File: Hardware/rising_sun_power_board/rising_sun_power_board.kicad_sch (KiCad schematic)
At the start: 30 parts, among them J1 POWER_IN, J2 Conn_01x03_Socket, J3 Conn_01x03_Socket, SW201 SW_Push, U1 ESP32, U2 MIC5219, U3 UA78M05IDCYR, U4 TXU0102DCUR

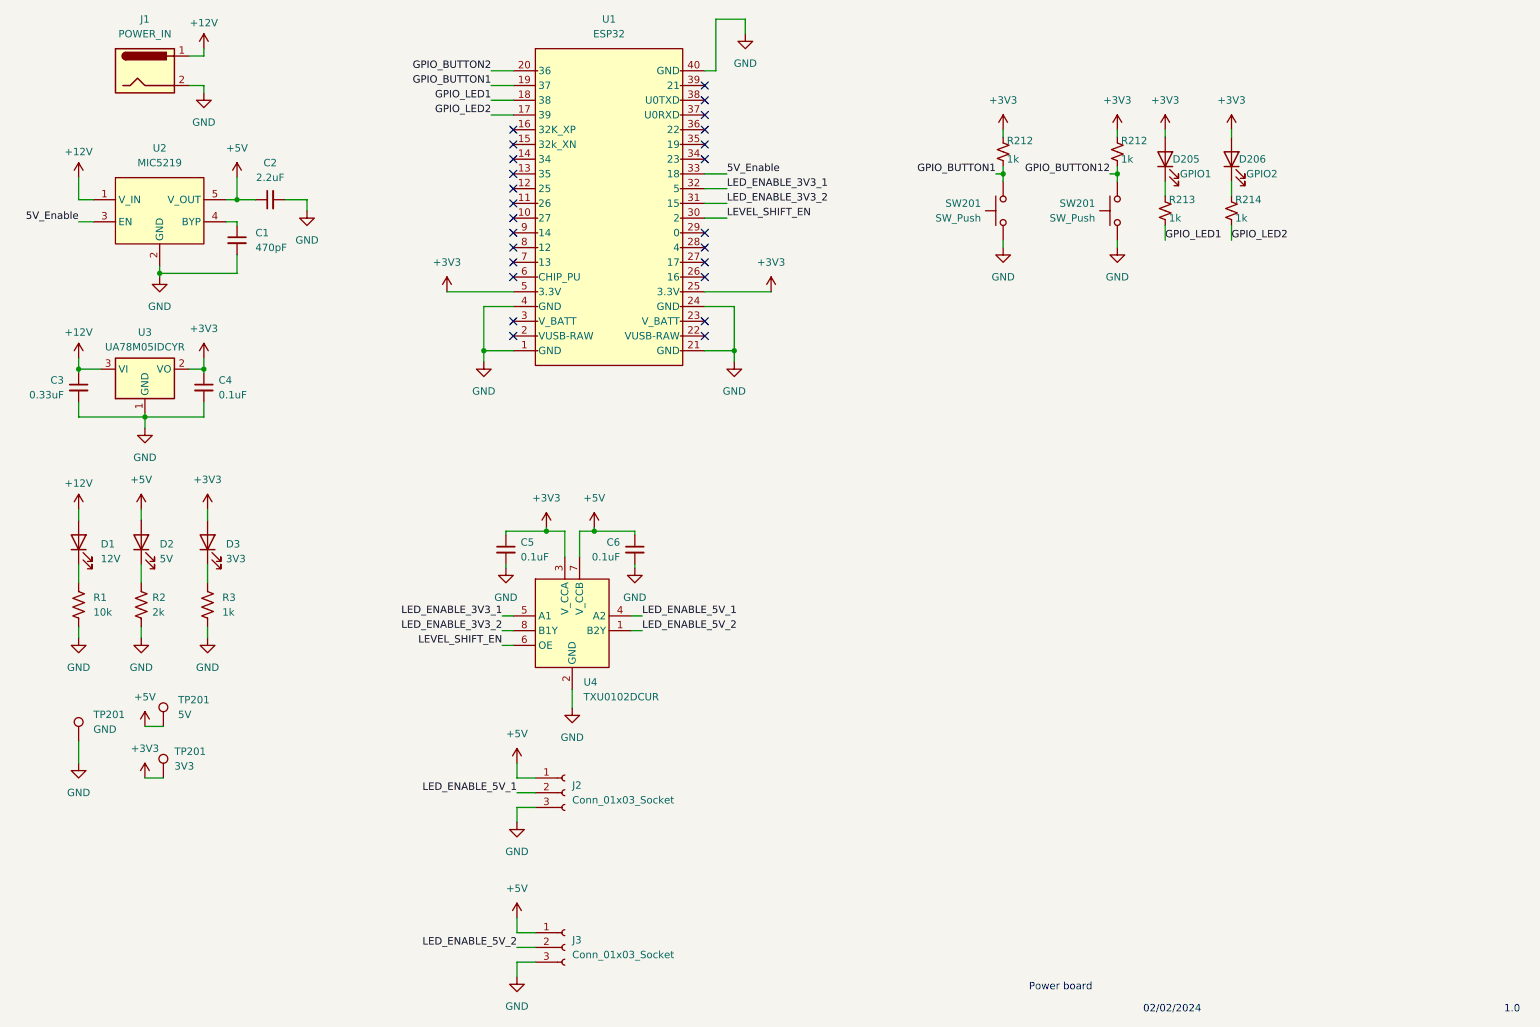
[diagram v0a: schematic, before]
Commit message: layout le done
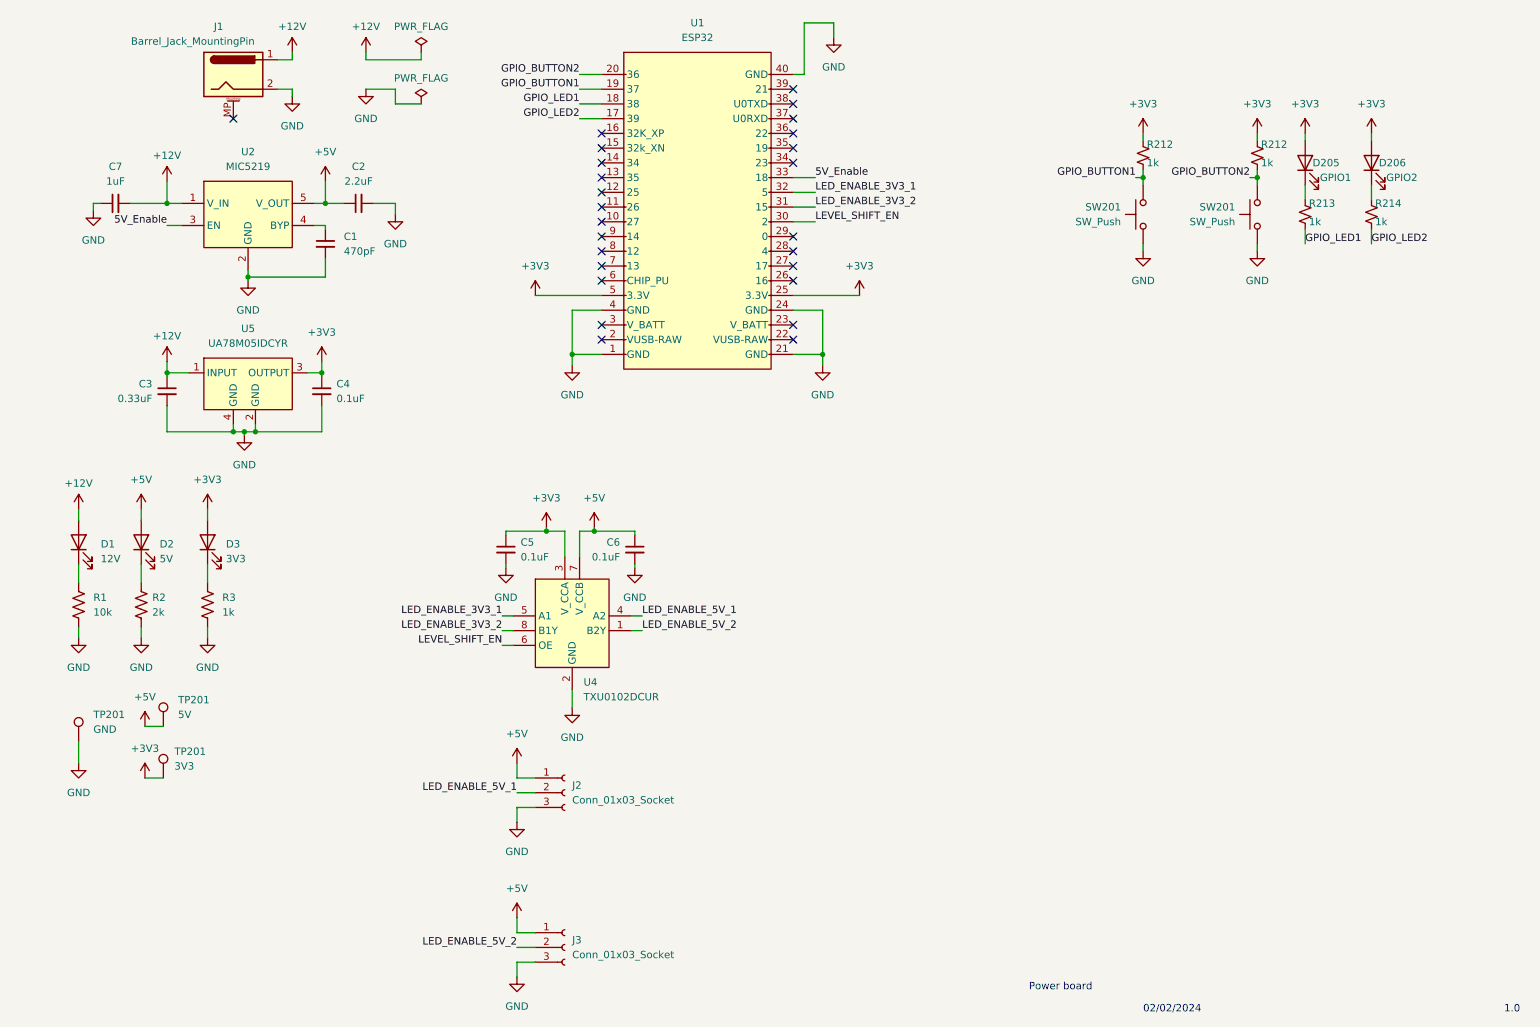
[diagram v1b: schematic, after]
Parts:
- removed J1: POWER_IN, Connector_BarrelJack:BarrelJack_Wuerth_6941xx301002, symbol Connector:Barrel_Jack
- removed U3: UA78M05IDCYR, Package_TO_SOT_SMD:SOT-223-3_TabPin2, symbol Regulator_Linear:AMS1117-3.3
- added C7: 1uF, Capacitor_SMD:C_0603_1608Metric, symbol Device:C_Small
- added J1: Barrel_Jack_MountingPin, custom_footprints:CUI_PJ-202A, symbol Connector:Barrel_Jack_MountingPin
- added U5: UA78M05IDCYR, Package_TO_SOT_SMD:SOT-223, symbol customLibrary:uA78M33
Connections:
- net GPIO_BUTTON12 is gone; now on net GPIO_BUTTON2: R212.2, SW201.1
- net +12V: now also C7.2, J1.1, U5.1 (INPUT)
- net +3V3: now also U5.3 (OUTPUT)
- net GND: now also C7.1, J1.2, U5.2 (GND), U5.4 (GND)
- no-connect marks 25 -> 26
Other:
- moved on the sheet: C1, C2, C3, C4, D205, D206, R212, R213, R214, SW201, U1, U2
